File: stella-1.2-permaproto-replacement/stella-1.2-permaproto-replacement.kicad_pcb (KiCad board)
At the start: 2 copper layers, 158 x 51 mm, 15 parts, among them J1 Conn_01x03, J2 Conn_01x04, SW1 RotaryEncoder_Switch, SW2 SW_Push, U1 Eyespi Breakout, U2 RTC, U3 MiniBoost, U4 GPS Breakout, U5 SD Reader

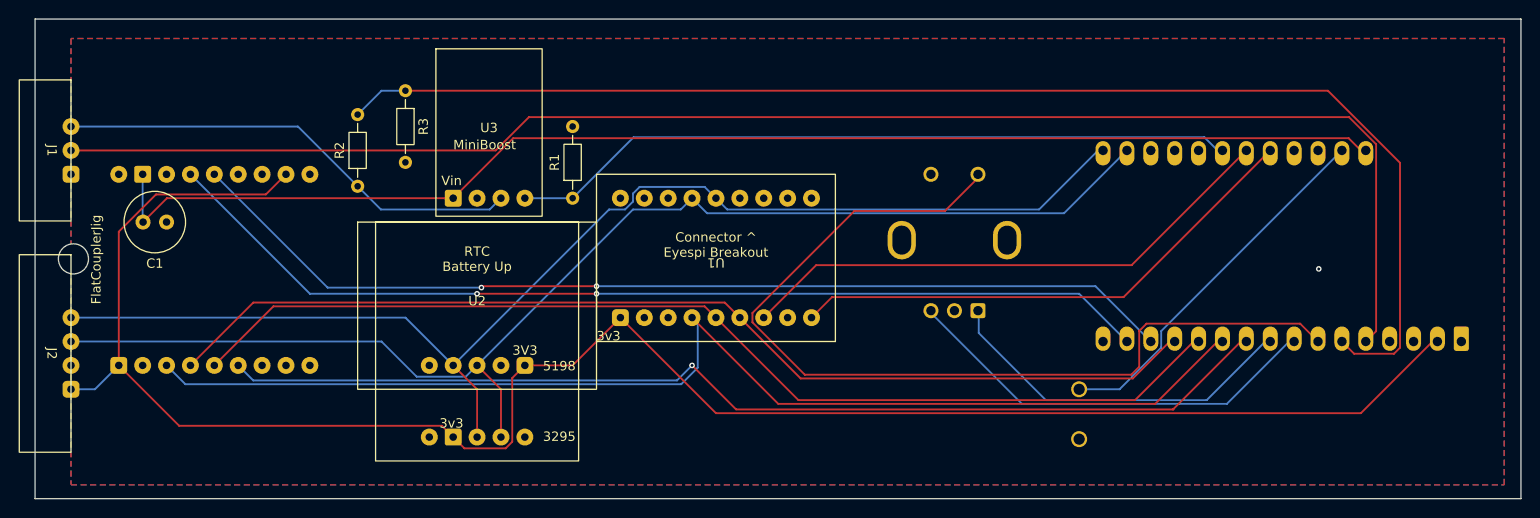
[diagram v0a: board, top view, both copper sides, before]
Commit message: Incorporate build fixes in base (size, pins, gnd plane thermal)
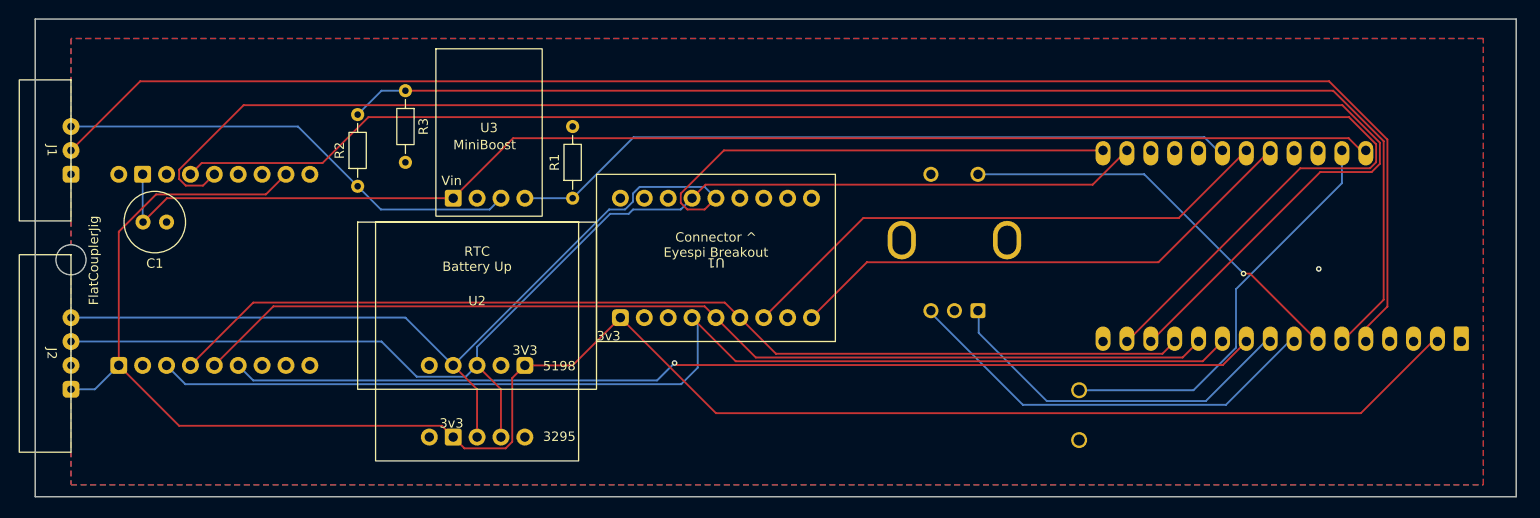
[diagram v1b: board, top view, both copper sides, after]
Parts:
- moved FlatCouplerJig 0.28 mm to (83.8, 100.5)
- moved SW2 0.10 mm to (191.0, 114.4)
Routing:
- net Net-(A1-RX/IO16): track 107.1 -> 172.1 mm, vias 2 -> 0
- net Net-(A1-TX/IO17): track 106.9 -> 166.1 mm, vias 2 -> 0
- net Net-(A1-I34/A2): track 98.7 -> 43.5 mm, vias 0 -> 1
- net /I2C_SDA: track 132.0 -> 140.5 mm
- net Net-(A1-DAC1/A1): track 141.7 -> 135.5 mm
- net Net-(A1-DAC2/A0): track 164.4 -> 169.6 mm
- net Net-(A1-EN): track 39.5 -> 44.2 mm
- net Net-(A1-IO4/A5): track 113.5 -> 109.8 mm
- net /SPI_SCK: track 126.6 -> 122.8 mm
- net /SPI_MOSI: track 114.0 -> 110.2 mm
- net /SPI_MISO: track 112.4 -> 110.2 mm
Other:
- board size 158 x 51 mm -> 157.5 x 50.8 mm
- board text added: "Stella-1.2 Base Permaproto Replacement PCB v0.1.1 2026 Layout by Nathan Eloe Should line up with original permaproto component placement"
- board text removed: "Stella-1.2 Base Permaproto Replacement PCB v0.1.0 2026 Layout by Nathan Eloe Should line up with original permaproto component placement"
